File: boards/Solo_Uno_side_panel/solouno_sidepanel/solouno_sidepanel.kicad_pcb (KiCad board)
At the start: 2 copper layers, 20 x 72 mm, 10 parts, among them CN1 CAN Front, CN2 CAN Back

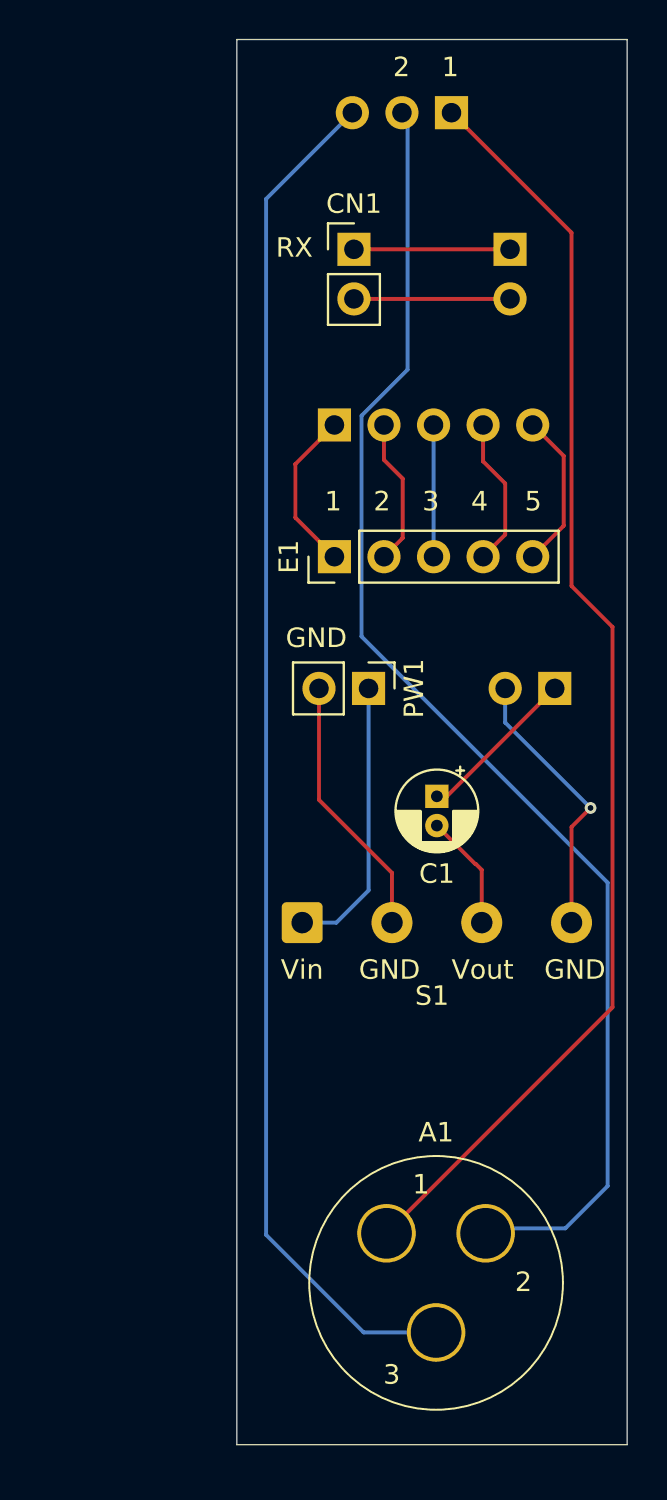
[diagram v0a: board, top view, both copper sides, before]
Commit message: Updated Solon
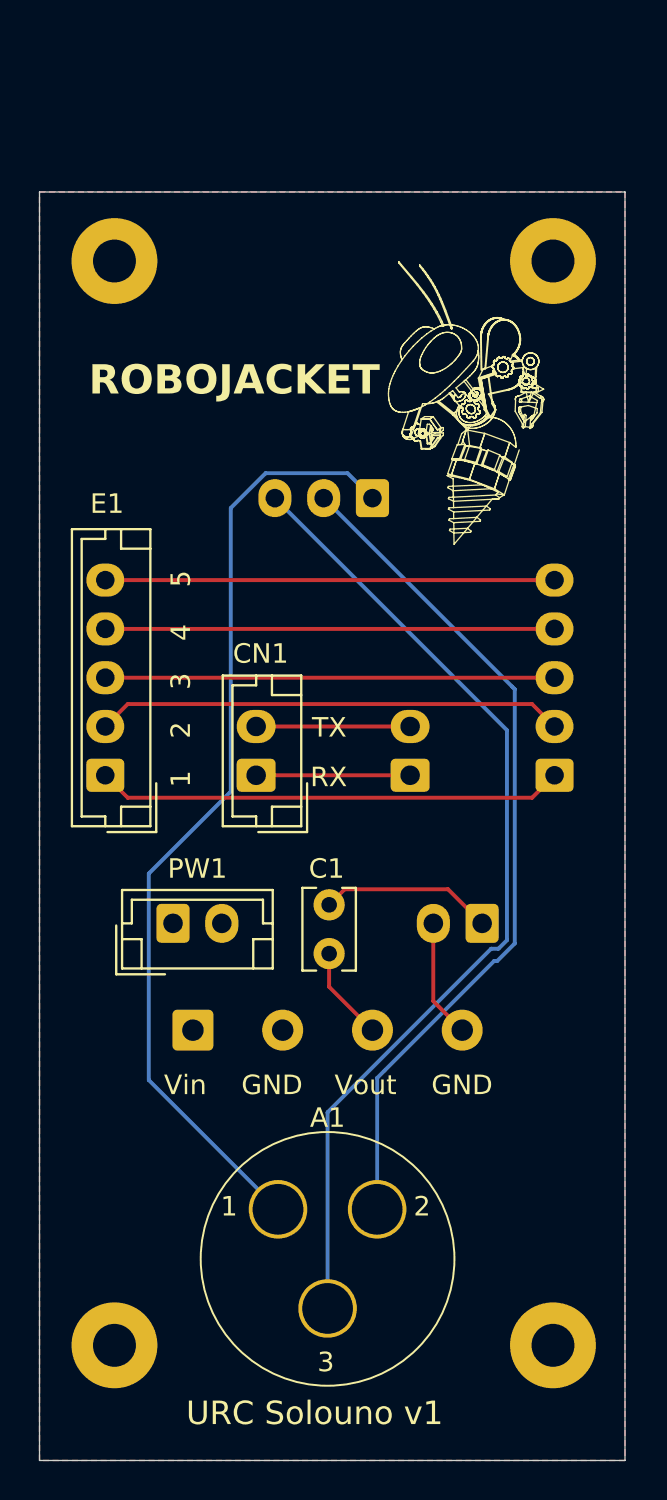
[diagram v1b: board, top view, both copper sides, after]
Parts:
- added hole1: MountingHole_2.2mm_M2_Pad, MountingHole:MountingHole_2.2mm_M2_Pad, F.Cu at (153.4, 159.9)
- added hole2: MountingHole_2.2mm_M2_Pad, MountingHole:MountingHole_2.2mm_M2_Pad, F.Cu at (131.0, 159.9)
- added hole3: MountingHole_2.2mm_M2_Pad, MountingHole:MountingHole_2.2mm_M2_Pad, F.Cu at (131.0, 104.3)
- added hole4: MountingHole_2.2mm_M2_Pad, MountingHole:MountingHole_2.2mm_M2_Pad, F.Cu at (153.4, 104.3)
- A2: footprint Connector_PinHeader_2.54mm:PinHeader_1x03_P2.54mm_Vertical -> Connector_JST:JST_EH_B3B-EH-A_1x03_P2.50mm_Vertical
- C1: footprint Capacitor_THT:CP_Radial_D4.0mm_P1.50mm -> Capacitor_THT:C_Rect_L4.0mm_W2.5mm_P2.50mm
- CN1, CN2, PW1, PW2: footprint Connector_PinHeader_2.54mm:PinHeader_1x02_P2.54mm_Vertical -> Connector_JST:JST_EH_B2B-EH-A_1x02_P2.50mm_Vertical
- E1, E2: footprint Connector_PinHeader_2.54mm:PinHeader_1x05_P2.54mm_Vertical -> Connector_JST:JST_EH_B5B-EH-A_1x05_P2.50mm_Vertical
- moved CN2 27.4 mm to (146.1, 130.7), turned to 90 degrees
- moved CN1 27.4 mm to (138.2, 130.7), turned to 90 degrees
- moved E2 21.2 mm to (153.5, 130.7), turned to 90 degrees
- moved A2 20.2 mm to (144.2, 116.5), turned to 180 degrees
- moved E1 16.2 mm to (130.5, 130.7)
- moved PW1 15.7 mm to (134.0, 138.3), turned to 0 degrees
- moved PW2 12.6 mm to (149.8, 138.3), turned to 180 degrees
- moved S1 7.86 mm to (135.0, 143.8)
- moved C1 7.84 mm to (142.0, 137.3)
- moved A1 5.69 mm to (141.9, 155.5)
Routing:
- net Net-(A2-Pin_2): track 68.6 -> 43.5 mm
- net Net-(A2-Pin_3): track 71.2 -> 50.5 mm
- net Net-(A2-Pin_1): track 67.3 -> 48.9 mm
- net Net-(E1-Pin_2): track 7.55 -> 24.0 mm
- net Net-(E1-Pin_3): track 6.75 -> 23.0 mm
- net Net-(E1-Pin_1): track 8.41 -> 24.0 mm
- net Net-(E1-Pin_4): track 7.69 -> 23.0 mm
- net Net-(E1-Pin_5): track 8.07 -> 23.0 mm
- net +28V: track 14.9 -> 0.00 mm
- net GND: track 13.5 -> 0.00 mm
- net Net-(PW2-Pin_2): track 14.4 -> 6.09 mm, vias 1 -> 0
- net Net-(S1-Pin_3): track 5.94 -> 4.84 mm
- net Net-(PW2-Pin_1): track 8.33 -> 8.90 mm
- added copper zone on F.Cu, net +28V
- added copper zone on B.Cu, net GND
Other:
- board size 20 x 72 mm -> 30 x 65 mm
- board text added: "ROBOJACKET"
- board text added: "TX"
- board text added: "URC Solouno v1"

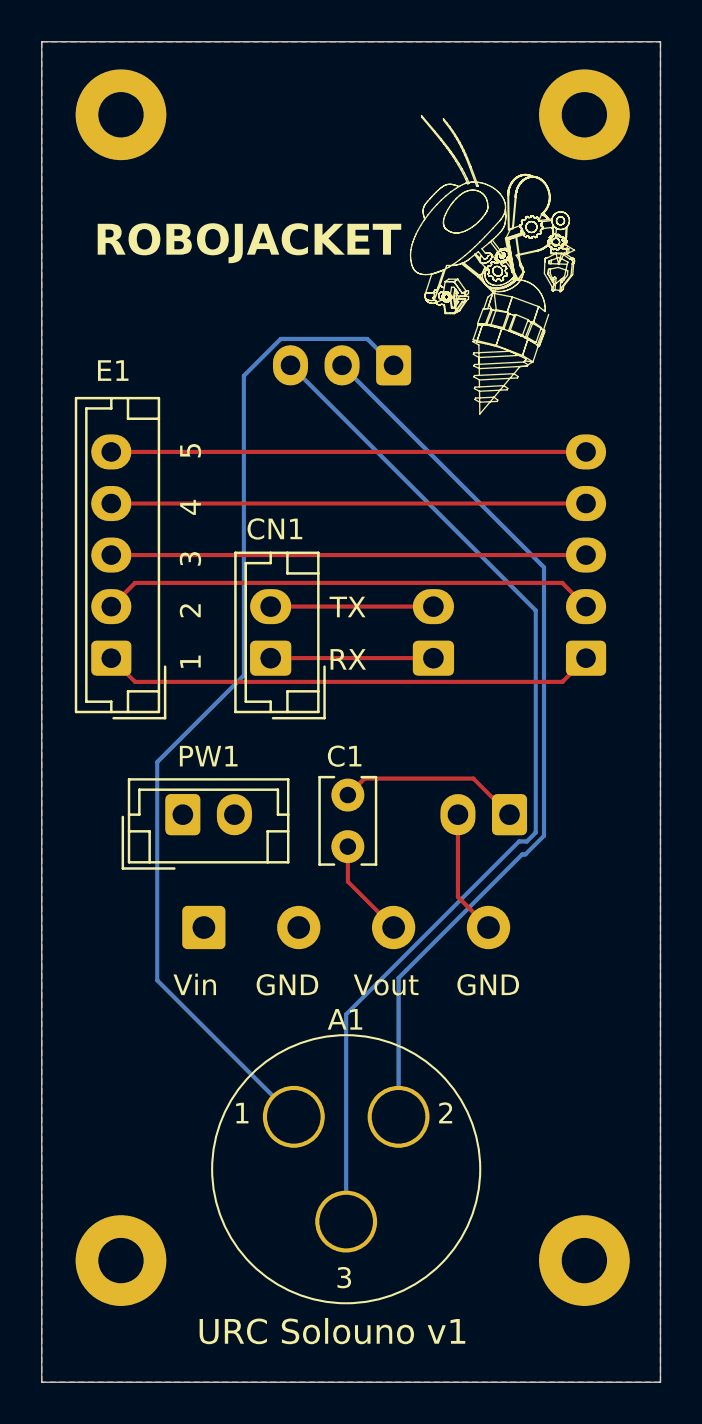
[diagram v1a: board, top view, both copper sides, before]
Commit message: side panel with Gerber
waiting for final aviation dimensions
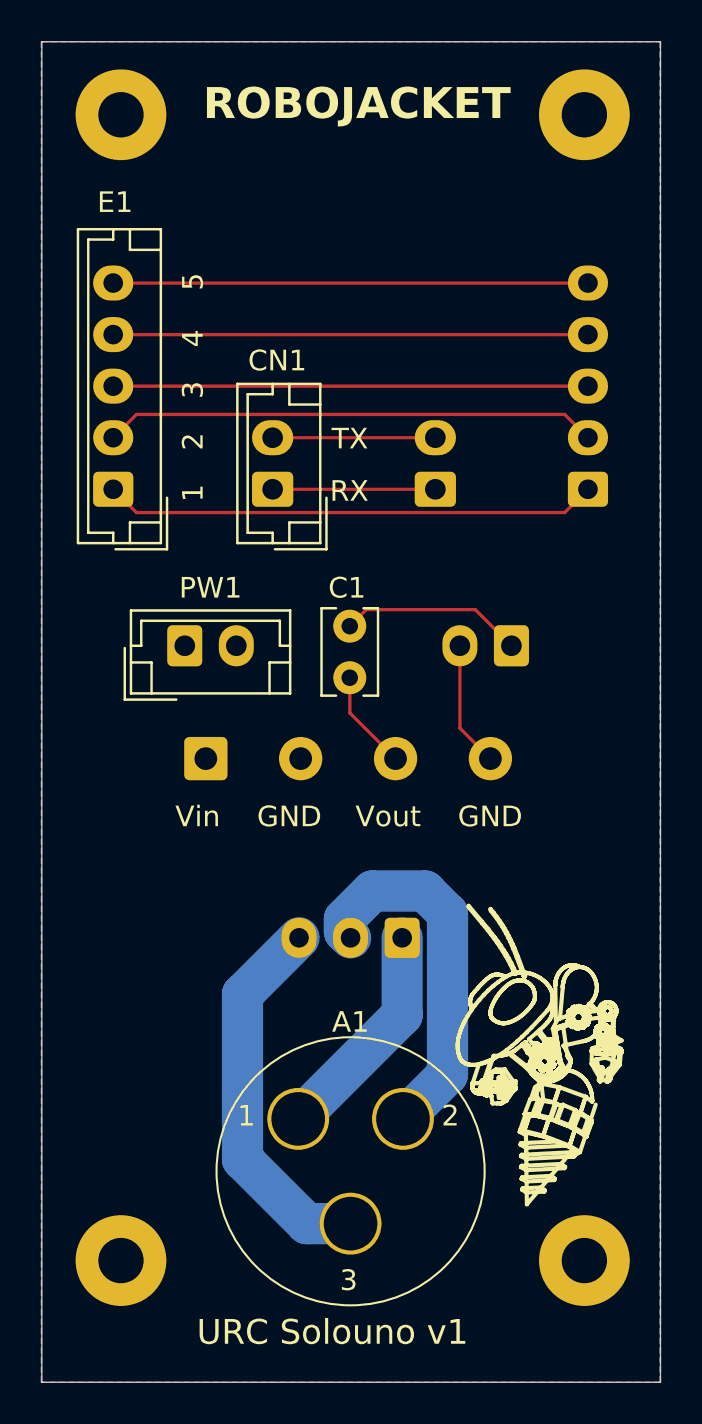
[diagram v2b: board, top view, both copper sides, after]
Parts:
- moved A2 27.8 mm to (144.6, 144.3)
- moved C1 8.19 mm to (142.1, 129.1)
- moved PW1 8.19 mm to (134.1, 130.1)
- moved PW2 8.19 mm to (149.9, 130.1)
- moved S1 8.19 mm to (135.1, 135.6)
- moved CN1 8.19 mm to (138.3, 122.5)
- moved CN2 8.19 mm to (146.2, 122.5)
- moved E1 8.19 mm to (130.6, 122.5)
- moved E2 8.19 mm to (153.6, 122.5)
- moved A1 0.24 mm to (142.1, 155.6)
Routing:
- net Net-(A2-Pin_1): track 48.9 -> 10.9 mm
- net Net-(A2-Pin_3): track 50.5 -> 18.4 mm
- net Net-(A2-Pin_2): track 43.5 -> 17.9 mm

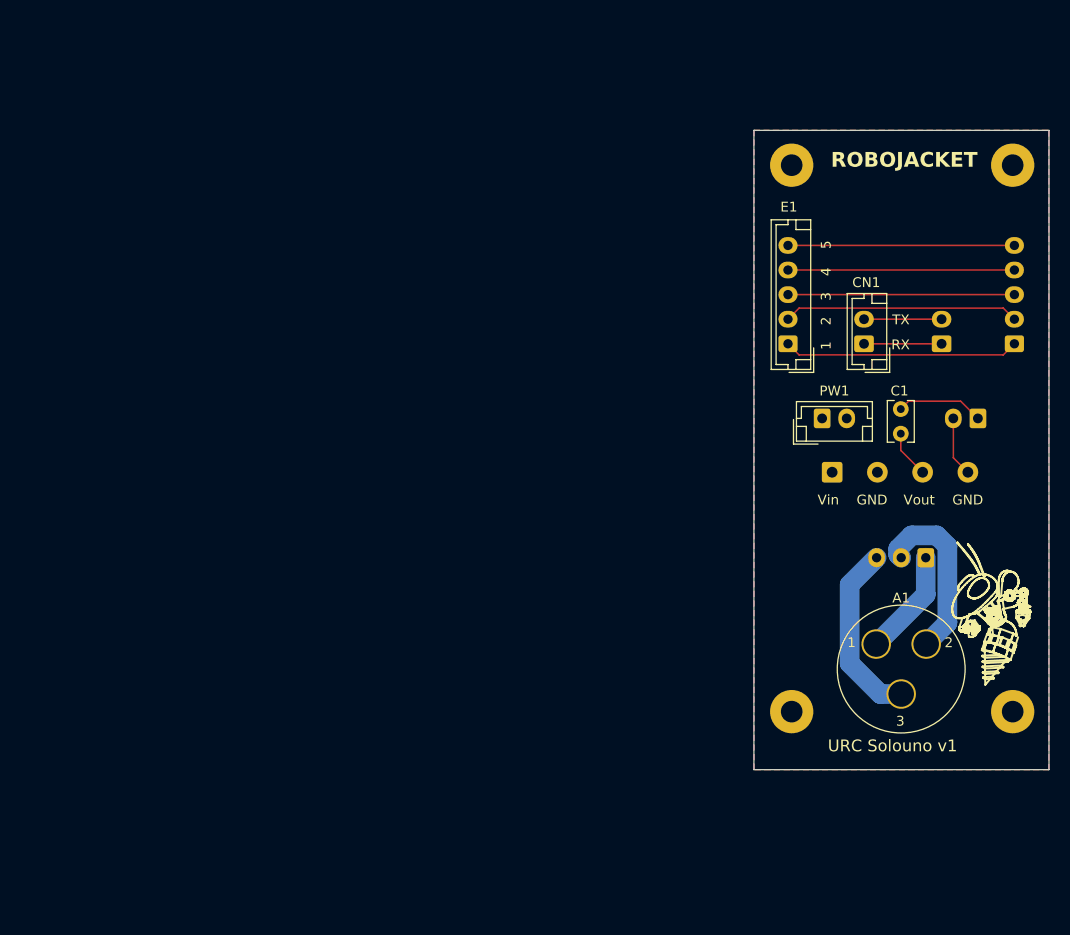
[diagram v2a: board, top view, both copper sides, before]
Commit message: side panel
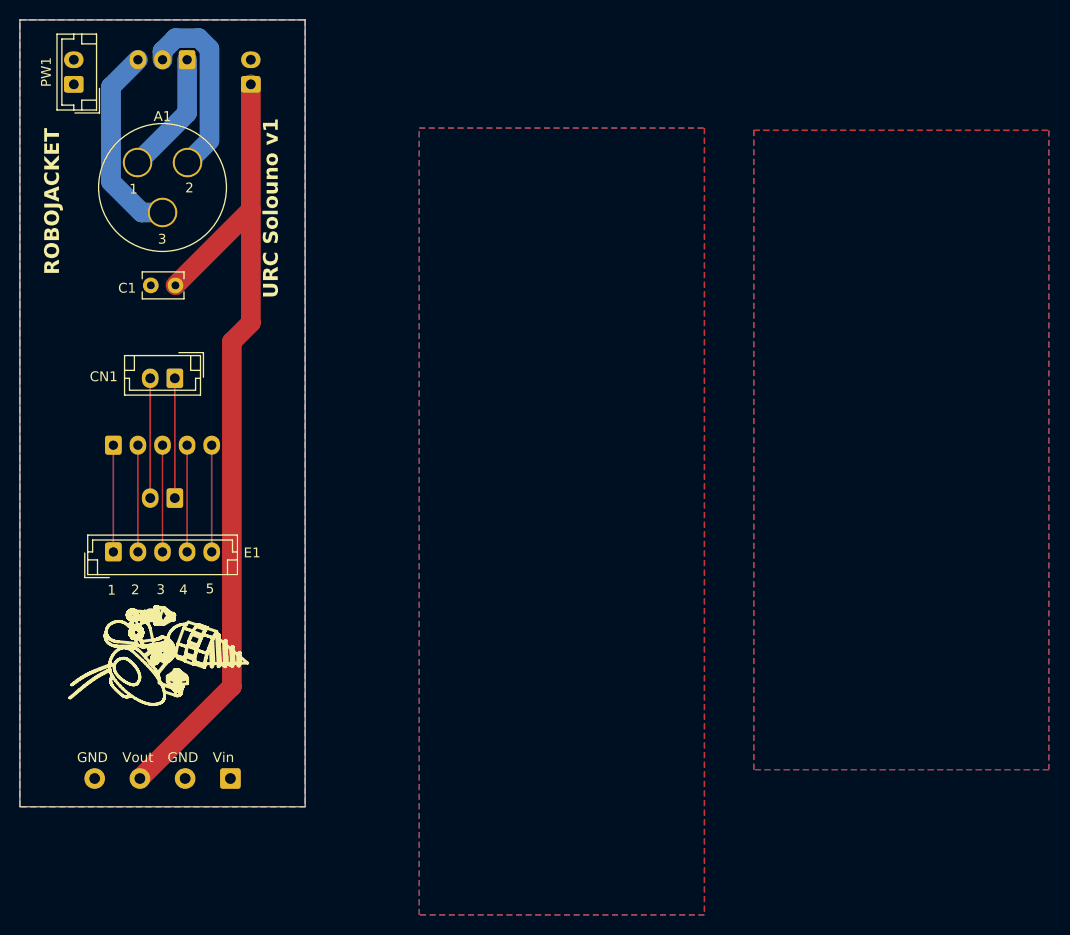
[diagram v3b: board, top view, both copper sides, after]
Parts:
- removed hole1, hole2, hole3, hole4: MountingHole_2.2mm_M2_Pad, MountingHole:MountingHole_2.2mm_M2_Pad
- moved E2 92.2 mm to (62.0, 132.8), turned to 0 degrees
- moved A2 90.6 mm to (69.5, 93.6)
- moved A1 89.7 mm to (67.0, 106.6)
- moved PW1 83.3 mm to (58.0, 96.1), turned to 90 degrees
- moved PW2 81.4 mm to (76.0, 96.1), turned to 90 degrees
- moved CN2 79.5 mm to (68.3, 138.2), turned to 180 degrees
- moved C1 74.8 mm to (68.3, 116.6), turned to 180 degrees
- moved E1 71.8 mm to (62.0, 143.7), turned to 0 degrees
- moved CN1 70.2 mm to (68.3, 126.0), turned to 180 degrees
- moved S1 68.7 mm to (73.9, 166.7), turned to 180 degrees
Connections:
- C1 pad 2: Net-(S1-Pin_3) -> GND
- PW2 pad 2: Net-(PW2-Pin_2) -> GND
- S1 pad 3: Net-(S1-Pin_3) -> Net-(PW2-Pin_1)
- S1 pad 4: Net-(PW2-Pin_2) -> GND
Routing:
- net Net-(PW2-Pin_1): track 8.90 -> 86.1 mm
- net Net-(E1-Pin_2): track 24.0 -> 10.8 mm
- net Net-(E1-Pin_1): track 24.0 -> 10.8 mm
- net Net-(E1-Pin_5): track 23.0 -> 10.8 mm
- net Net-(E1-Pin_4): track 23.0 -> 10.8 mm
- net Net-(E1-Pin_3): track 23.0 -> 10.8 mm
- net Net-(PW2-Pin_2): track 6.09 -> 0.00 mm
- net Net-(S1-Pin_3): track 4.84 -> 0.00 mm
- net Net-(CN1-Pin_2): track 7.89 -> 12.2 mm
- net Net-(CN1-Pin_1): track 7.89 -> 12.2 mm
- net Net-(A2-Pin_1): track 10.9 -> 12.5 mm
- net Net-(A2-Pin_3): track 18.4 -> 20.1 mm
- net Net-(A2-Pin_2): track 17.9 -> 19.1 mm
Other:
- board size 30 x 65 mm -> 29 x 80 mm
- board text removed: "RX"
- board text removed: "TX"
